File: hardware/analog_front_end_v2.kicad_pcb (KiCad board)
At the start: 4 copper layers, 142.9 x 41.4 mm, 101 parts, among them J1 Conn_Coaxial, J3 Conn_01x01_Socket, J4 Conn_01x01_Socket, U1 ADL5531, U10 MAX6002, U11 LP2985-5.0, U12 MAX2606, U13 PAT1220-C-0DB, U14 LP2985-5.0, U15 BFP540ESD, U16 BFP540ESD, U17 LP2985-3.3, U18 PAT1220-C-0DB, U19 PAT1220-C-0DB, U2 ADL5531, U20 PAT1220-C-0DB, U21 PAT1220-C-0DB, U3 ADL5531, U4 ADL5531, U5 LP2985-1.8, U6 MCP33131, U7 PAT1220-C-0DB, U8 ADL5531, U9 PMOD 2x6

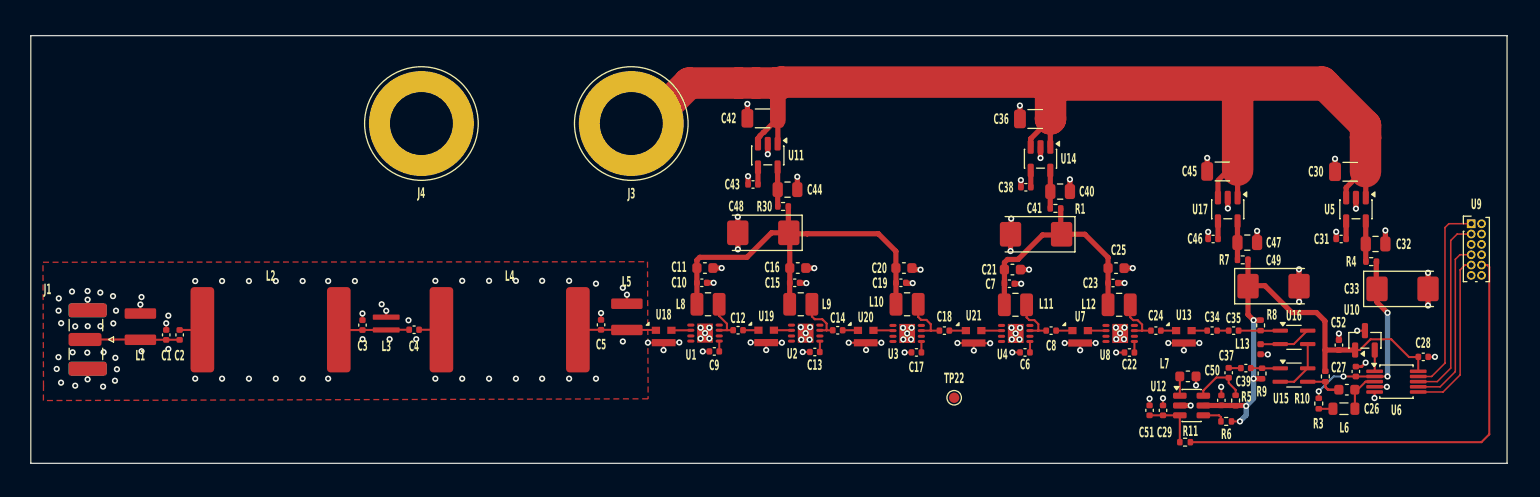
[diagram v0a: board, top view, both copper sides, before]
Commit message: Latest KiCAD9.0 project file
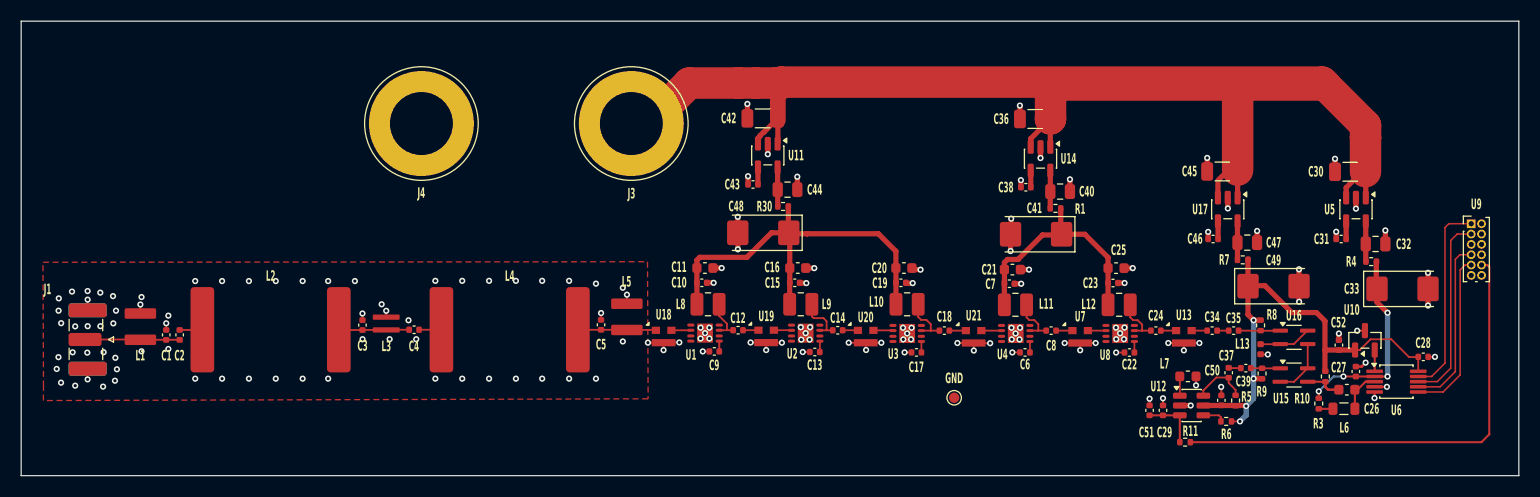
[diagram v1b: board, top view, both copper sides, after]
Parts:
- renumbered TP22 to GND
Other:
- board size 142.9 x 41.4 mm -> 145 x 44 mm
- board text added: "Decisions: Dimensions: 145mm x 44mm Use Coplanar Waveguide for RF filter section for more confined EM fields Use 0.6x0.3 vias Use 7mil trace for CPW section with 4mil gap to coplanar ground (Standard PCB manufacturer limit) assuming 1ounce copper, 0.1mm high prepreg, 4.6 dielectric constant Use 1mm via distance (2xgap) Use 2mm between vias horizontally Use 7mil for microstrip for around 50ohm imp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"
- board text removed: "TODO: Add solid GND planes on layers 2/3 Ground via stitching Decisions: Use Coplanar Waveguide for RF filter section for more confined EM fields Use 0.6x0.3 vias Use 8mil trace with 0.05mm airgap assuming 1ounce copper, 4.6 dielectric constant Use 1mm via distance (2xgap) Use 2mm between vias horizontally for microstrip with solid groundplane in layers 2,3 oriented horizontally for EM fields Use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"
